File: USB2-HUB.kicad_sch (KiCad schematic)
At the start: 23 parts, among them J17 USB_OTG, U12 TLV71311PDBV, U20 FSUSB42MUX, U4 TPD4EUSB30, U6 TUSB4041I, Y3 24MHz

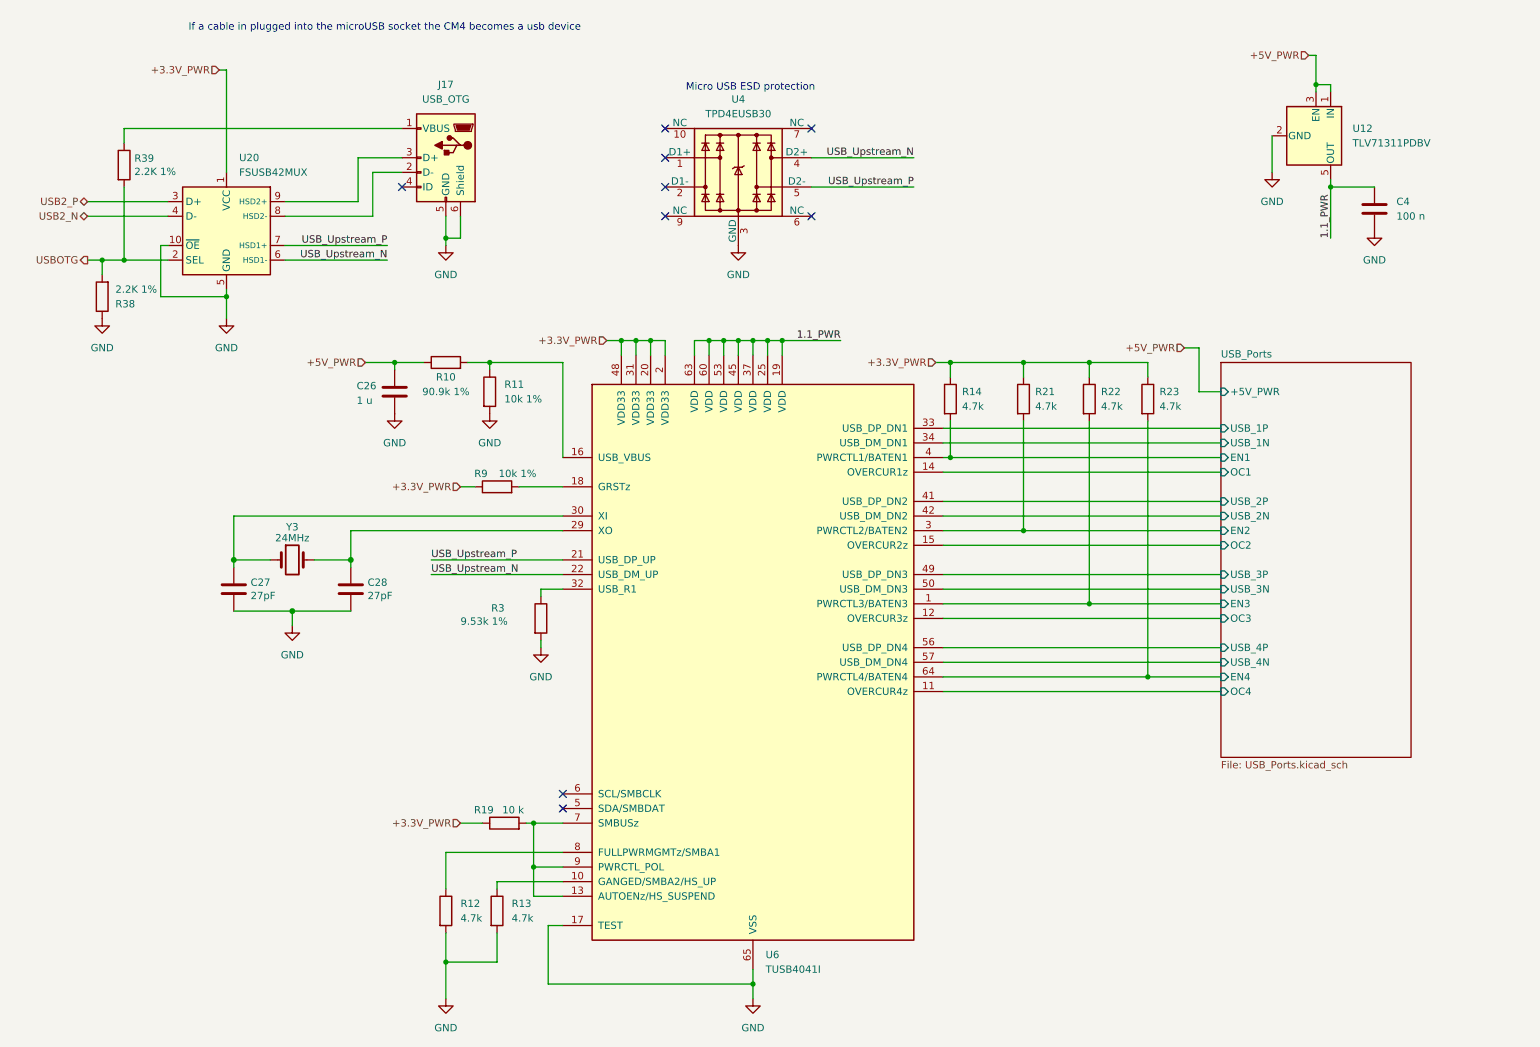
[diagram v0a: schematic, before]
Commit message: small changes for ravi
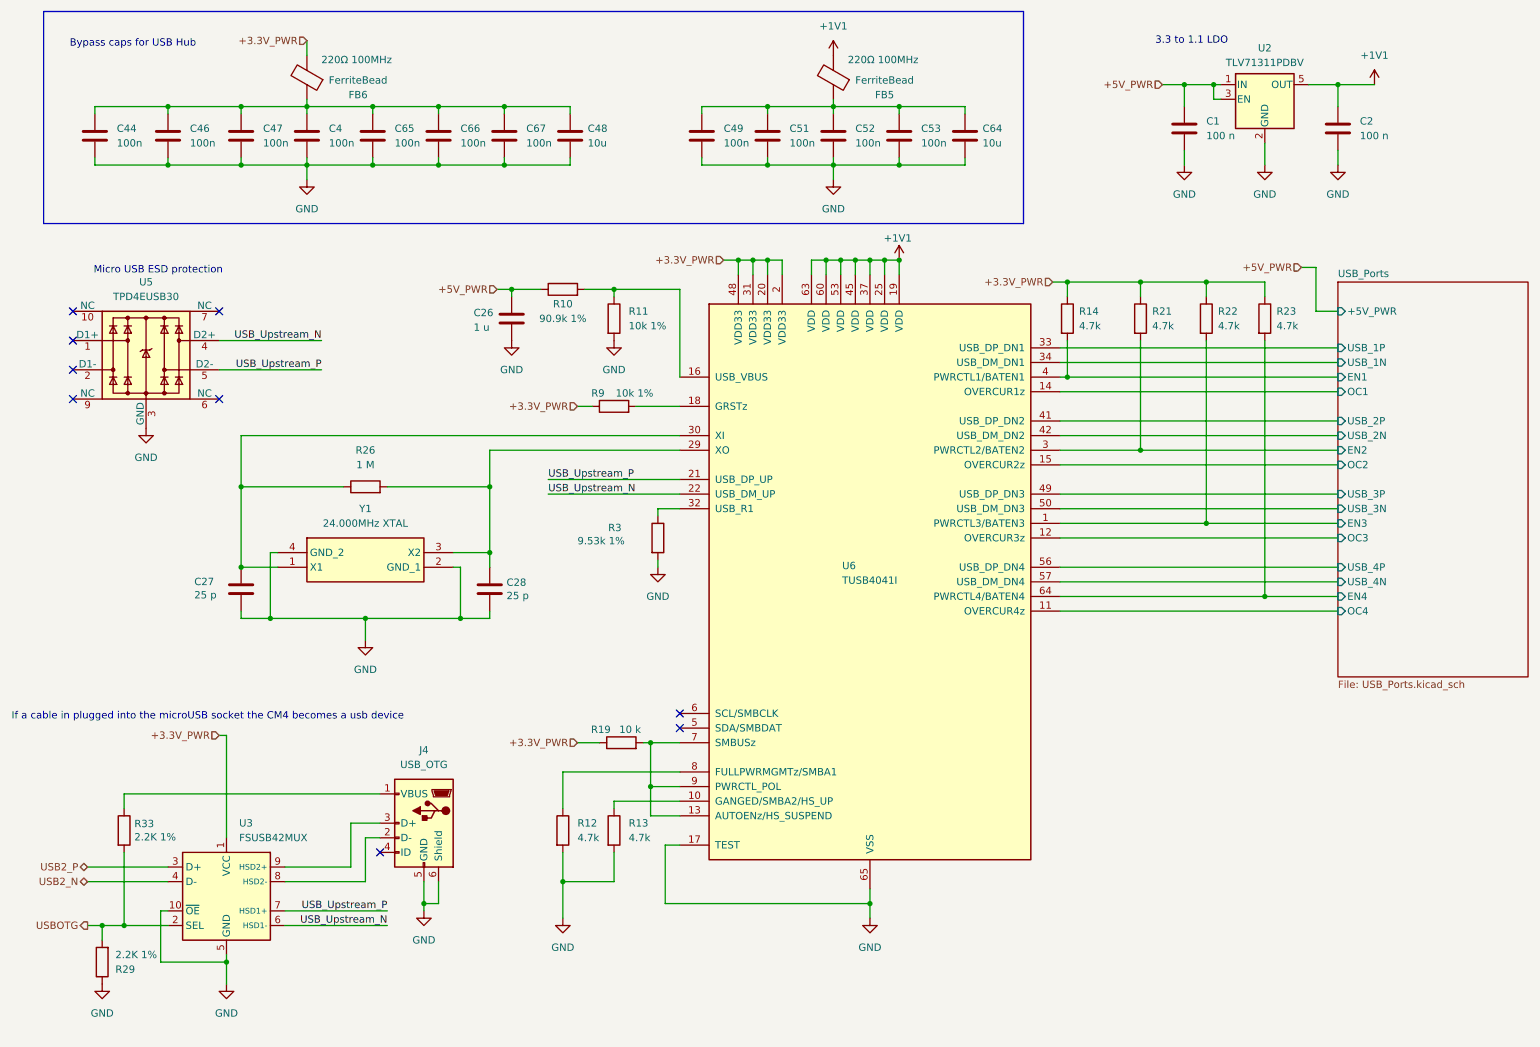
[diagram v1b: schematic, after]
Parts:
- removed J17: USB_OTG, symbol Connector:USB_OTG
- removed R38, R39: 2.2K 1%, Resistor_SMD:R_0402_1005Metric, symbol Device:R
- removed U12: TLV71311PDBV, Package_TO_SOT_SMD:SOT-23-5, symbol Regulator_Linear:TLV71311PDBV
- removed U20: FSUSB42MUX, Package_SO:MSOP-10_3x3mm_P0.5mm, symbol Interface_USB:FSUSB42MUX
- removed U4: TPD4EUSB30, Package_SON:USON-10_2.5x1.0mm_P0.5mm, symbol Power_Protection:TPD4EUSB30
- removed Y3: 24MHz, Crystal:Crystal_SMD_HC49-SD, symbol Device:Crystal
- added C1, C2: 100 n, symbol Device:C
- added C44, C46, C47, C49, C51, C52, C53, C65, C66, C67: 100n, symbol Device:C
- added C48, C64: 10u, symbol Device:C
- added FB5, FB6: FerriteBead, symbol Device:FerriteBead
- added J4: USB_OTG, symbol Connector:USB_OTG
- added R26: 1 M, symbol Device:R
- added R29, R33: 2.2K 1%, Resistor_SMD:R_0402_1005Metric, symbol Device:R
- added U2: TLV71311PDBV, Package_TO_SOT_SMD:SOT-23-5, symbol Regulator_Linear:TLV71311PDBV
- added U3: FSUSB42MUX, Package_SO:MSOP-10_3x3mm_P0.5mm, symbol Interface_USB:FSUSB42MUX
- added U5: TPD4EUSB30, Package_SON:USON-10_2.5x1.0mm_P0.5mm, symbol Power_Protection:TPD4EUSB30
- added Y1: 24.000MHz XTAL, ABM8AIG25000MHZ122ZT3, symbol ABM8AIG-24.000MHZ-12-2Z-T3:ABM8AIG-24.000MHZ-12-2Z-T3
- C27, C28: value 27pF -> 25 p
- C4: value 100 n -> 100n
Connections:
- net +3.3V_PWR: now also FB6.2, U3.1 (VCC)
- net +5V_PWR: now also C1.1, U2.1 (IN), U2.3 (EN)
- net GND: now also C1.2, C2.2, C44.2, C46.2, C47.2, C48.2, C49.2, C51.2, C52.2, C53.2, C64.2, C65.2, C66.2, C67.2, J4.5 (GND), J4.6 (Shield), R29.1, U2.2 (GND), U3.10 (~{OE}), U3.5 (GND), U5.3 (GND), U5.8 (GND), Y1.2 (GND_1), Y1.4 (GND_2)
- net USB2_N: now also U3.4 (D-)
- net USB2_P: now also U3.3 (D+)
- net USBOTG: now also R29.2, R33.2, U3.2 (SEL)
- net USB_Upstream_N: now also U3.6 (HSD1-), U5.4 (D2+)
- net USB_Upstream_P: now also U3.7 (HSD1+), U5.5 (D2-)
- net at C27.1, U6.30 (XI): now also R26.1, Y1.1 (X1)
- net at C28.1, U6.29 (XO): now also R26.2, Y1.3 (X2)
- net 1.1_PWR renamed +1V1
- net +1V1: now also C2.1, FB5.2, U2.5 (OUT); no longer C4.1
- new net: C4.1, C44.1, C46.1, C47.1, C48.1, C65.1, C66.1, C67.1, FB6.1
- new net: J4.2 (D-), U3.8 (HSD2-)
- new net: J4.3 (D+), U3.9 (HSD2+)
- new net: C49.1, C51.1, C52.1, C53.1, C64.1, FB5.1
- new net: J4.1 (VBUS), R33.1
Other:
- note added: "3.3 to 1.1 LDO"
- note added: "Bypass caps for USB Hub"
- moved on the sheet: C26, C27, C28, R10, R11, R12, R13, R14, R19, R21, R22, R23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
